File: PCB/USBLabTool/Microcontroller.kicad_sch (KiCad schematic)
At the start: 17 parts, among them J1 Conn_01x06_Pin, J2 Conn_02x12_Odd_Even, SW1 SW_Push, U12 STM32H562VGTx, Y1 32.768kHz

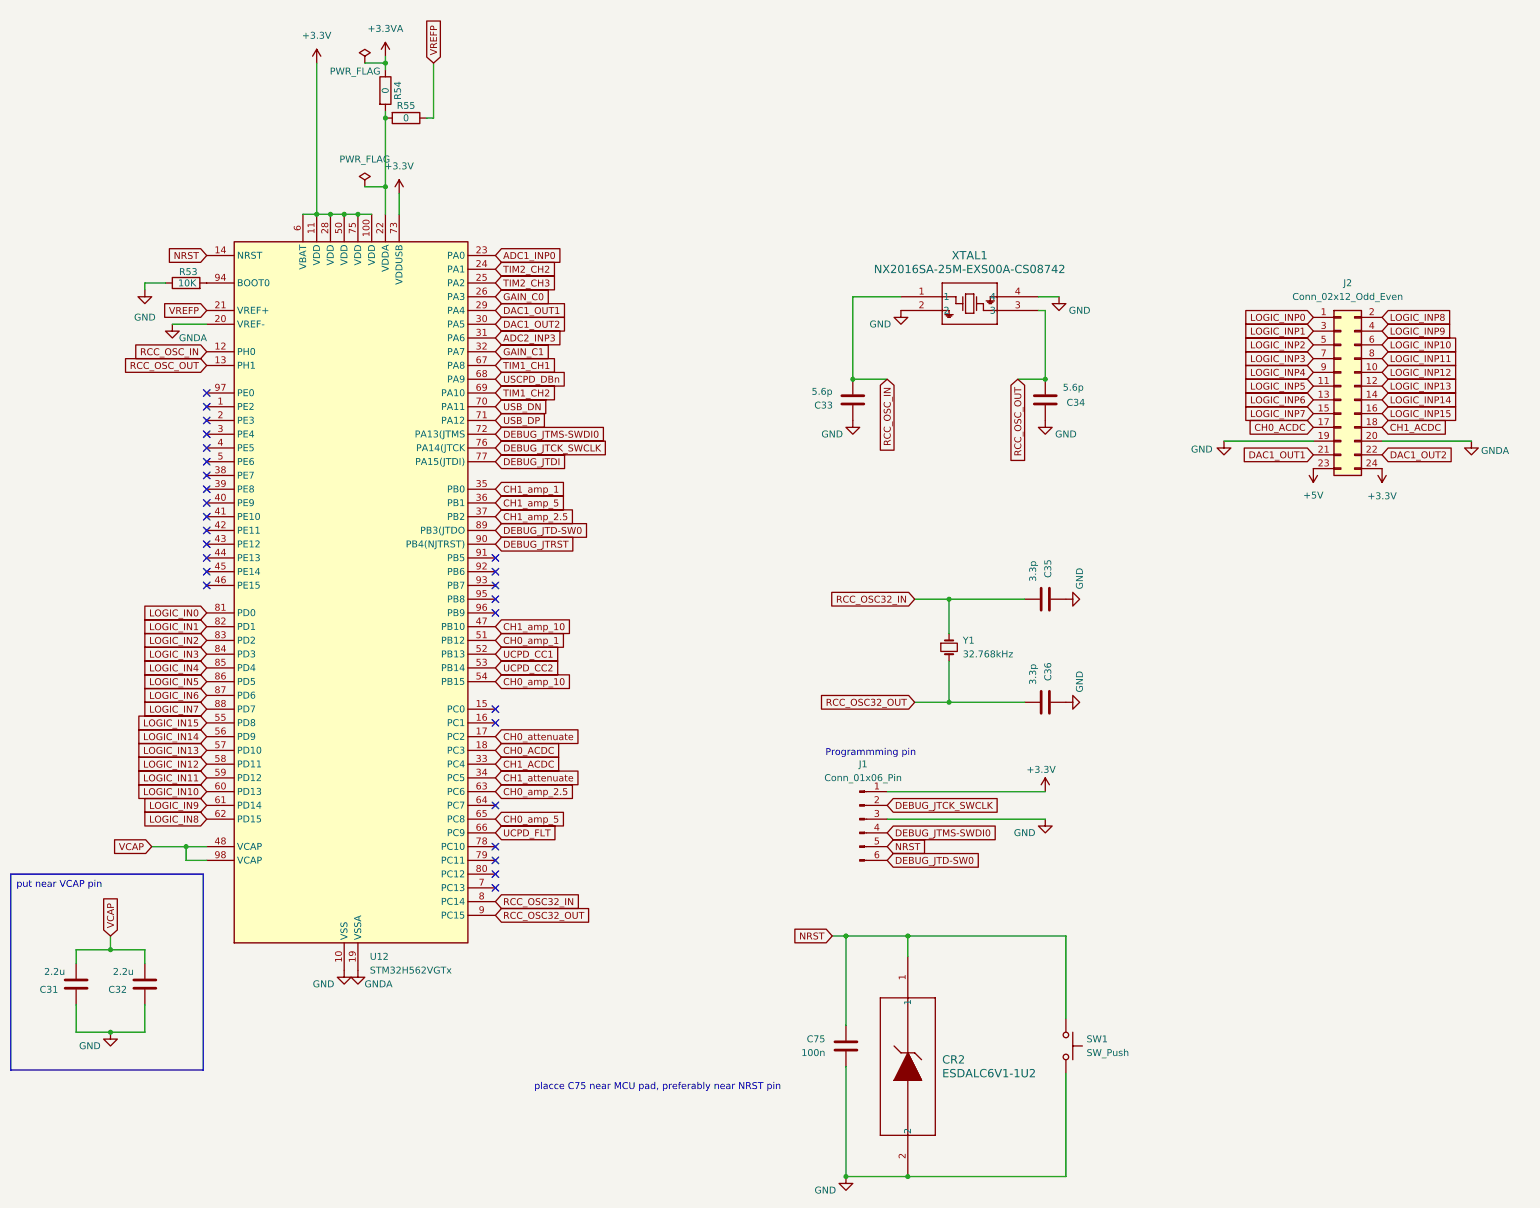
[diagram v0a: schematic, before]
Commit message: continue PCB layout
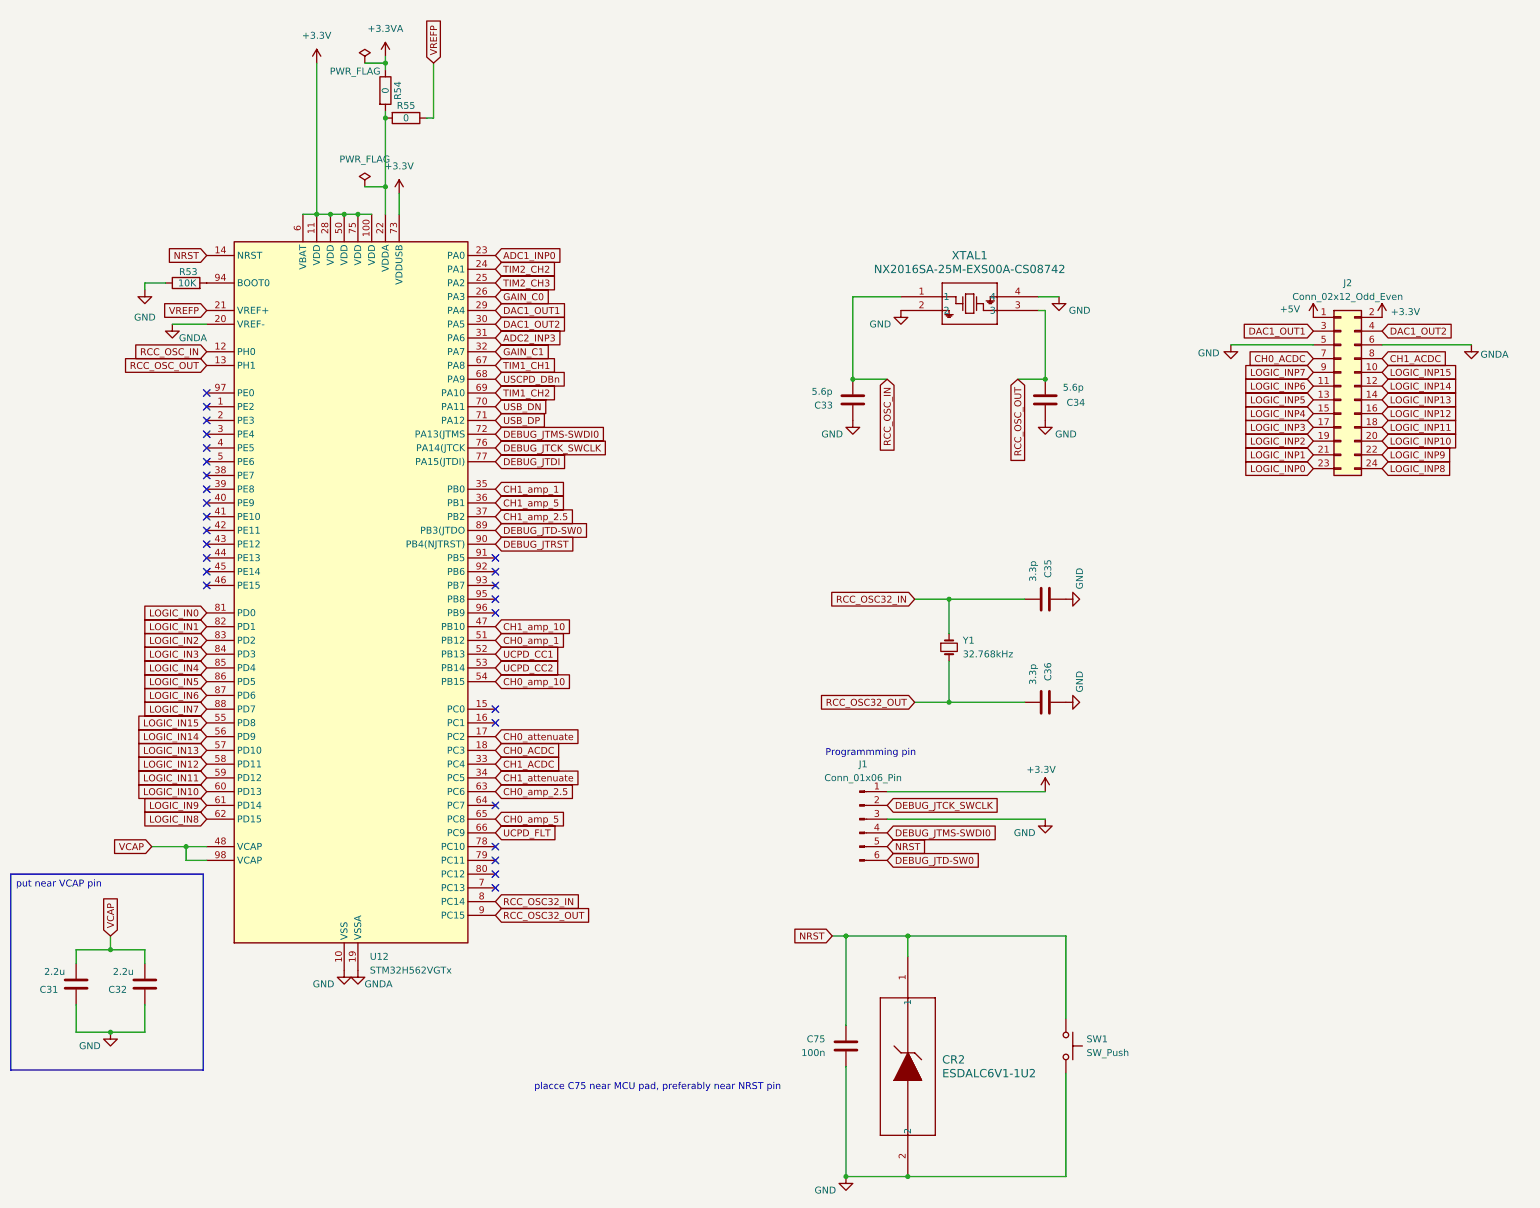
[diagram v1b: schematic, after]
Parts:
- J2: footprint Connector_JST:JST_PHD_S24B-PHDSS_2x12_P2.00mm_Horizontal -> userfp:OST_302-R241
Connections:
- net +3.3V: now also J2.2 (Pin_2); no longer J2.24 (Pin_24)
- net +5V: now also J2.1 (Pin_1); no longer J2.23 (Pin_23)
- net CH0_ACDC: now also J2.7 (Pin_7); no longer J2.17 (Pin_17)
- net CH1_ACDC: now also J2.8 (Pin_8); no longer J2.18 (Pin_18)
- net DAC1_OUT1: now also J2.3 (Pin_3); no longer J2.21 (Pin_21)
- net DAC1_OUT2: now also J2.4 (Pin_4); no longer J2.22 (Pin_22)
- net GND: now also J2.5 (Pin_5); no longer J2.19 (Pin_19)
- net GNDA: now also J2.6 (Pin_6); no longer J2.20 (Pin_20)
- net LOGIC_INP0: now also J2.23 (Pin_23); no longer J2.1 (Pin_1)
- net LOGIC_INP1: now also J2.21 (Pin_21); no longer J2.3 (Pin_3)
- net LOGIC_INP10: now also J2.20 (Pin_20); no longer J2.6 (Pin_6)
- net LOGIC_INP11: now also J2.18 (Pin_18); no longer J2.8 (Pin_8)
- net LOGIC_INP12: now also J2.16 (Pin_16); no longer J2.10 (Pin_10)
- net LOGIC_INP13: now also J2.14 (Pin_14); no longer J2.12 (Pin_12)
- net LOGIC_INP14: now also J2.12 (Pin_12); no longer J2.14 (Pin_14)
- net LOGIC_INP15: now also J2.10 (Pin_10); no longer J2.16 (Pin_16)
- net LOGIC_INP2: now also J2.19 (Pin_19); no longer J2.5 (Pin_5)
- net LOGIC_INP3: now also J2.17 (Pin_17); no longer J2.7 (Pin_7)
- net LOGIC_INP4: now also J2.15 (Pin_15); no longer J2.9 (Pin_9)
- net LOGIC_INP5: now also J2.13 (Pin_13); no longer J2.11 (Pin_11)
- net LOGIC_INP6: now also J2.11 (Pin_11); no longer J2.13 (Pin_13)
- net LOGIC_INP7: now also J2.9 (Pin_9); no longer J2.15 (Pin_15)
- net LOGIC_INP8: now also J2.24 (Pin_24); no longer J2.2 (Pin_2)
- net LOGIC_INP9: now also J2.22 (Pin_22); no longer J2.4 (Pin_4)
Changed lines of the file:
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@@
 (kicad_sch
-	(version 20231120)
+	(version 20250114)
 	(generator "eeschema")
-	(generator_version "8.0")
+	(generator_version "9.0")
 	(paper "A3")

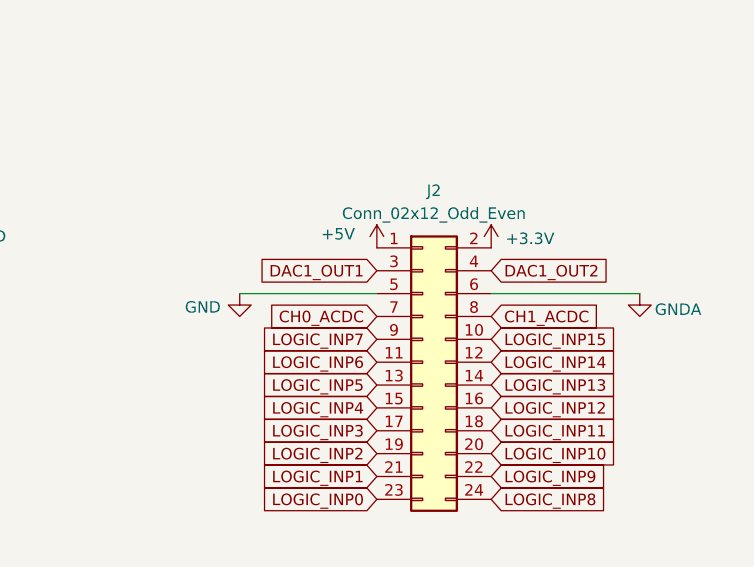
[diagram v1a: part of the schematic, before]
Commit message: some very small wirings, and layout
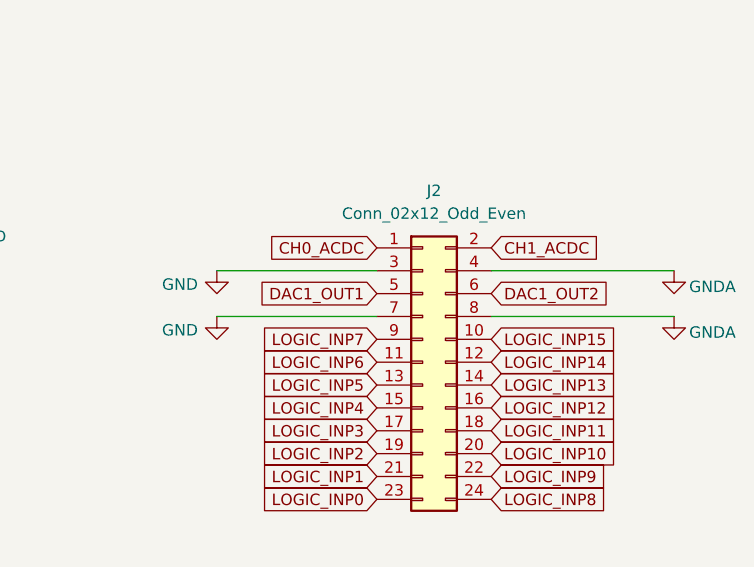
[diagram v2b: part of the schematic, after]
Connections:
- net +5V is gone; now on net CH0_ACDC: J2.1 (Pin_1)
- net +3.3V: no longer J2.2 (Pin_2)
- net CH0_ACDC: no longer J2.7 (Pin_7)
- net CH1_ACDC: now also J2.2 (Pin_2); no longer J2.8 (Pin_8)
- net DAC1_OUT1: now also J2.5 (Pin_5); no longer J2.3 (Pin_3)
- net DAC1_OUT2: now also J2.6 (Pin_6); no longer J2.4 (Pin_4)
- net GND: now also J2.3 (Pin_3), J2.7 (Pin_7); no longer J2.5 (Pin_5)
- net GNDA: now also J2.4 (Pin_4), J2.8 (Pin_8); no longer J2.6 (Pin_6)
